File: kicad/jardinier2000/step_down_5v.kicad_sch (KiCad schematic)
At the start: 14 parts, among them J2 VIN Reg, J8 5V, U3 TPS62933P

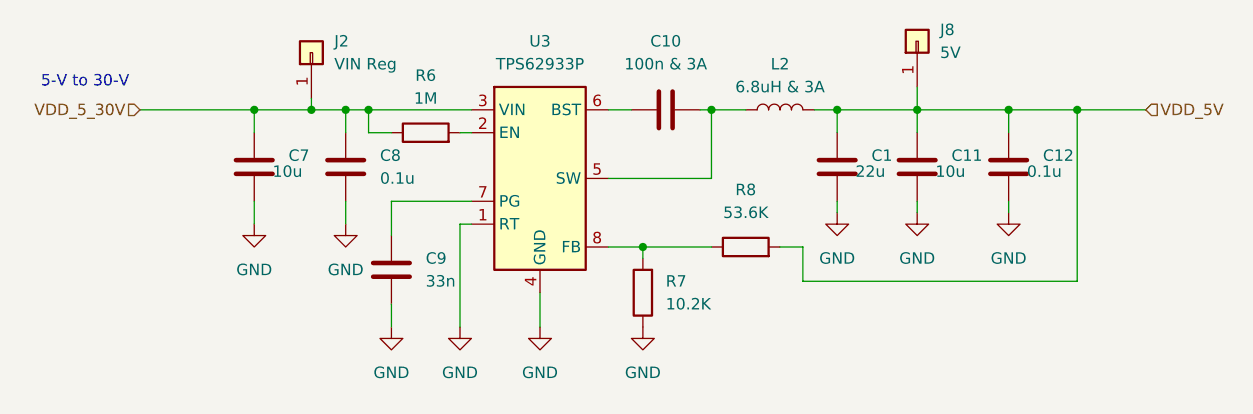
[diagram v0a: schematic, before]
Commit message: Updating schematics for v2
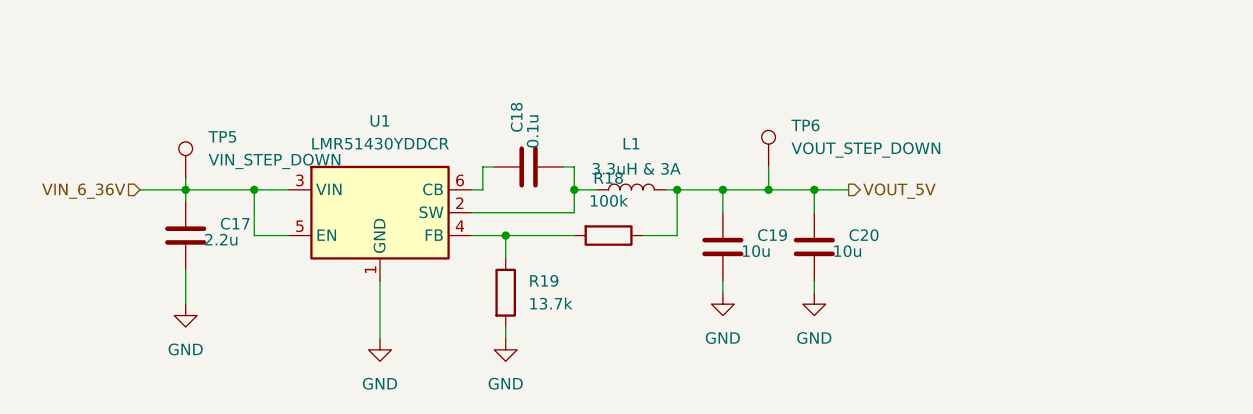
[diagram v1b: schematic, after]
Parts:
- removed C1: 22u, Capacitor_SMD:C_0805_2012Metric_Pad1.18x1.45mm_HandSolder, symbol Device:C
- removed C10: 100n & 3A, Capacitor_SMD:C_0805_2012Metric_Pad1.18x1.45mm_HandSolder, symbol Device:C
- removed C11, C7: 10u, Capacitor_SMD:C_0805_2012Metric_Pad1.18x1.45mm_HandSolder, symbol Device:C
- removed C12, C8: 0.1u, Capacitor_SMD:C_0805_2012Metric_Pad1.18x1.45mm_HandSolder, symbol Device:C
- removed C9: 33n, Capacitor_SMD:C_0805_2012Metric_Pad1.18x1.45mm_HandSolder, symbol Device:C
- removed J2: VIN Reg, Connector_PinHeader_1.00mm:PinHeader_1x01_P1.00mm_Vertical, symbol Connector_Generic:Conn_01x01
- removed J8: 5V, Connector_PinHeader_1.00mm:PinHeader_1x01_P1.00mm_Vertical, symbol Connector_Generic:Conn_01x01
- removed L2: 6.8uH & 3A, Inductor_SMD:L_1008_2520Metric_Pad1.43x2.20mm_HandSolder, symbol Device:L
- removed R6: 1M, Resistor_SMD:R_0805_2012Metric_Pad1.20x1.40mm_HandSolder, symbol Device:R
- removed R7: 10.2K, Resistor_SMD:R_0805_2012Metric_Pad1.20x1.40mm_HandSolder, symbol Device:R
- removed R8: 53.6K, Resistor_SMD:R_0805_2012Metric_Pad1.20x1.40mm_HandSolder, symbol Device:R
- removed U3: TPS62933P, Package_TO_SOT_SMD:SOT-583-8, symbol Regulator_Switching:TPS62933P
- added C17: 2.2u, Capacitor_SMD:C_0805_2012Metric_Pad1.18x1.45mm_HandSolder, symbol Device:C
- added C18: 0.1u, Capacitor_SMD:C_0805_2012Metric_Pad1.18x1.45mm_HandSolder, symbol Device:C
- added C19, C20: 10u, Capacitor_SMD:C_0805_2012Metric_Pad1.18x1.45mm_HandSolder, symbol Device:C
- added L1: 3.3uH & 3A, Inductor_SMD:L_Cenker_CKCS6028, symbol Device:L
- added R18: 100k, Resistor_SMD:R_0805_2012Metric_Pad1.20x1.40mm_HandSolder, symbol Device:R
- added R19: 13.7k, Resistor_SMD:R_0805_2012Metric_Pad1.20x1.40mm_HandSolder, symbol Device:R
- added TP5: VIN_STEP_DOWN, TestPoint:TestPoint_Pad_2.0x2.0mm, symbol Connector:TestPoint
- added TP6: VOUT_STEP_DOWN, TestPoint:TestPoint_Pad_2.0x2.0mm, symbol Connector:TestPoint
- added U1: LMR51430YDDCR, Package_TO_SOT_SMD:SOT-23-6, symbol Regulator_Switching:LMR51430
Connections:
- net GND: now also C17.2, C19.2, C20.2, R19.2, U1.1 (GND)
- new net: R18.2, R19.1, U1.4 (FB)
- new net: C18.2, L1.1, U1.2 (SW)
- new net: C18.1, U1.6 (CB)
- new net VIN_6_36V: C17.1, TP5.1, U1.3 (VIN), U1.5 (EN)
- new net VOUT_5V: C19.1, C20.1, L1.2, R18.1, TP6.1
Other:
- note removed: "5-V to 30-V"
